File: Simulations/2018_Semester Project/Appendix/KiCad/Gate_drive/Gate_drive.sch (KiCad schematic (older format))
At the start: 38 parts, among them J1 Inputs, J2 Gate:A, J3 VSS:A, J4 Gate:B, J5 VSS:B, Q1 PHPT60415NY, Q2 PHPT60415PY, Q3 BC846A, Q4 PHPT60415NY, Q5 PHPT60415PY, U1 L78L15ABUTR, U2 MGJ2D241509SC, U3 UCC20520, U4 MGJ2D241509SC

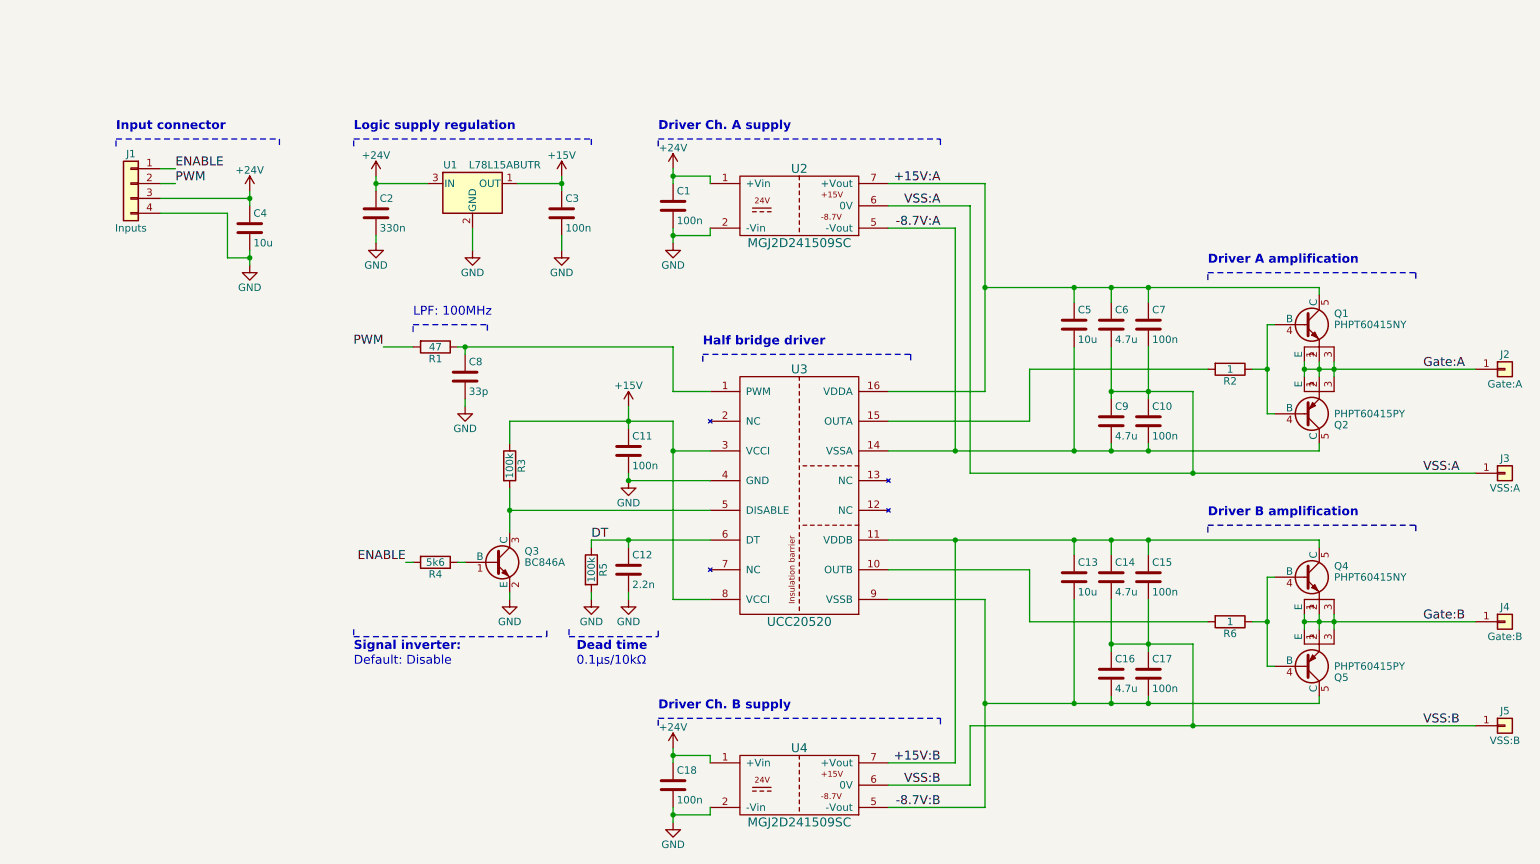
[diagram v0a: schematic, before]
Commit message: Data under light load
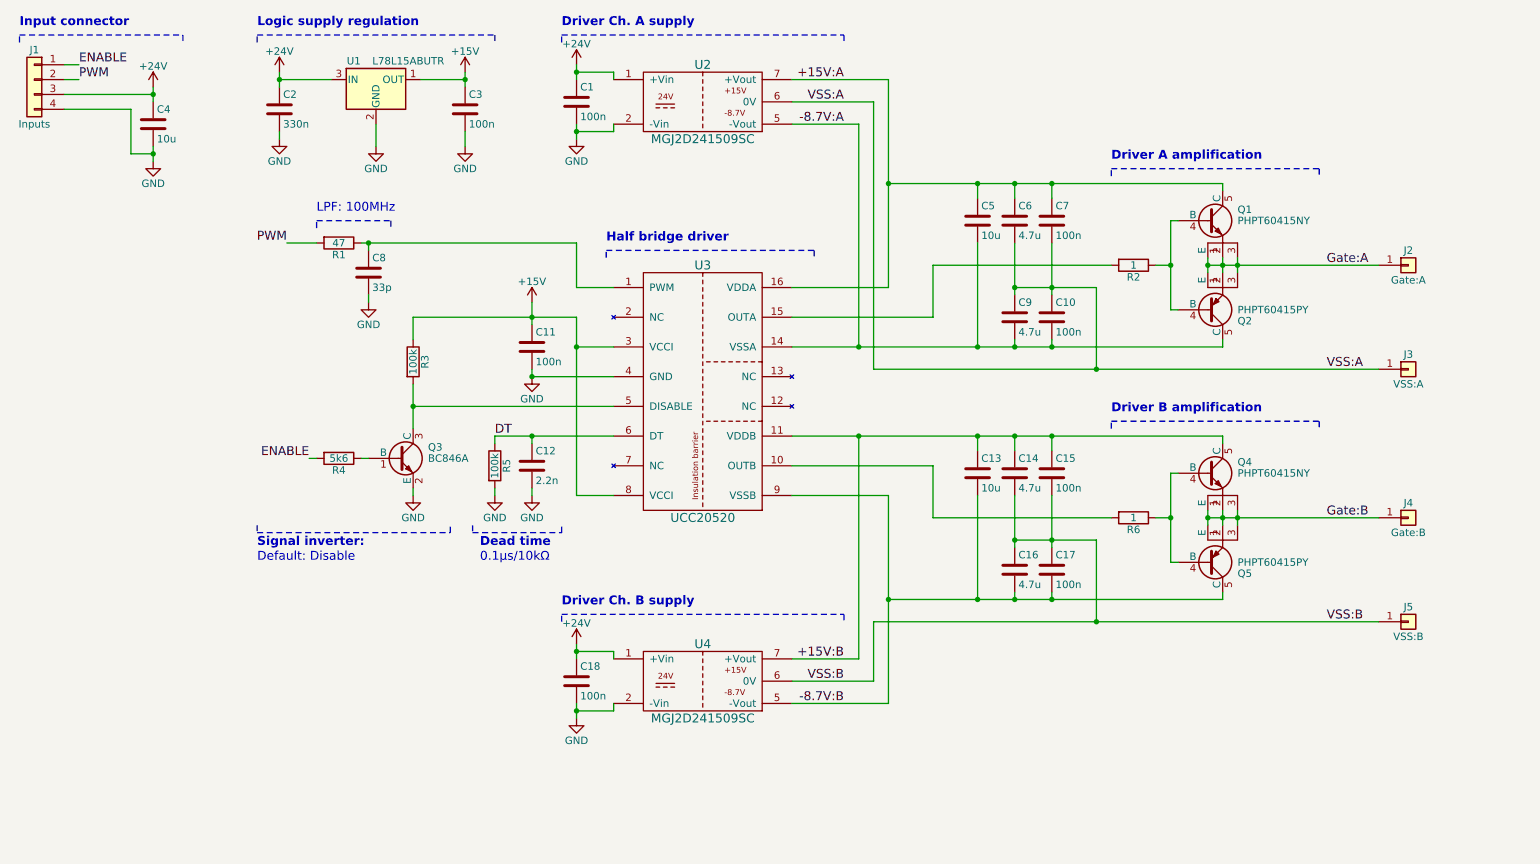
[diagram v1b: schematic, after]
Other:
- moved on the sheet: C1, C10, C11, C12, C13, C14, C15, C16, C17, C18, C2, C3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
